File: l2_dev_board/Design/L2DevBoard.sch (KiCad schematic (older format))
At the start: 18 parts, among them P101 CONN_10X2, P102 CONN_10X2, P103 CONN_10X2, P104 CONN_10X2, P105 CONN_10X2, P106 CONN_10X2, P107 CONN_10X2, P108 CONN_10X2, P109 CONN_10X2, P110 CONN_10X2, P111 CONN_10X2, P112 CONN_10X2, P113 CONN_10X2, P114 CONN_10X2, P115 CONN_10X2, U101 ASE_20MHZ

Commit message: missing header connector for 2 L2s. Find space!
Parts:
- added P?: CONN_10X2, symbol CONN_10X2
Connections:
- net GND: now also P102.19 (P19), P103.19 (P19), P108.19 (P19), P112.19 (P19), P113.11 (P11), P113.13 (P13), P113.15 (P15), P113.17 (P17), P113.19 (P19), P113.3 (P3), P113.5 (P5), P113.7 (P7), P113.9 (P9), P114.19 (P19), P115.1 (P1), P?.1 (P1), P?.11 (P11), P?.13 (P13), P?.15 (P15), P?.17 (P17), P?.19 (P19), P?.3 (P3), P?.5 (P5), P?.7 (P7), P?.9 (P9)
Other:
- moved on the sheet: P112, P113

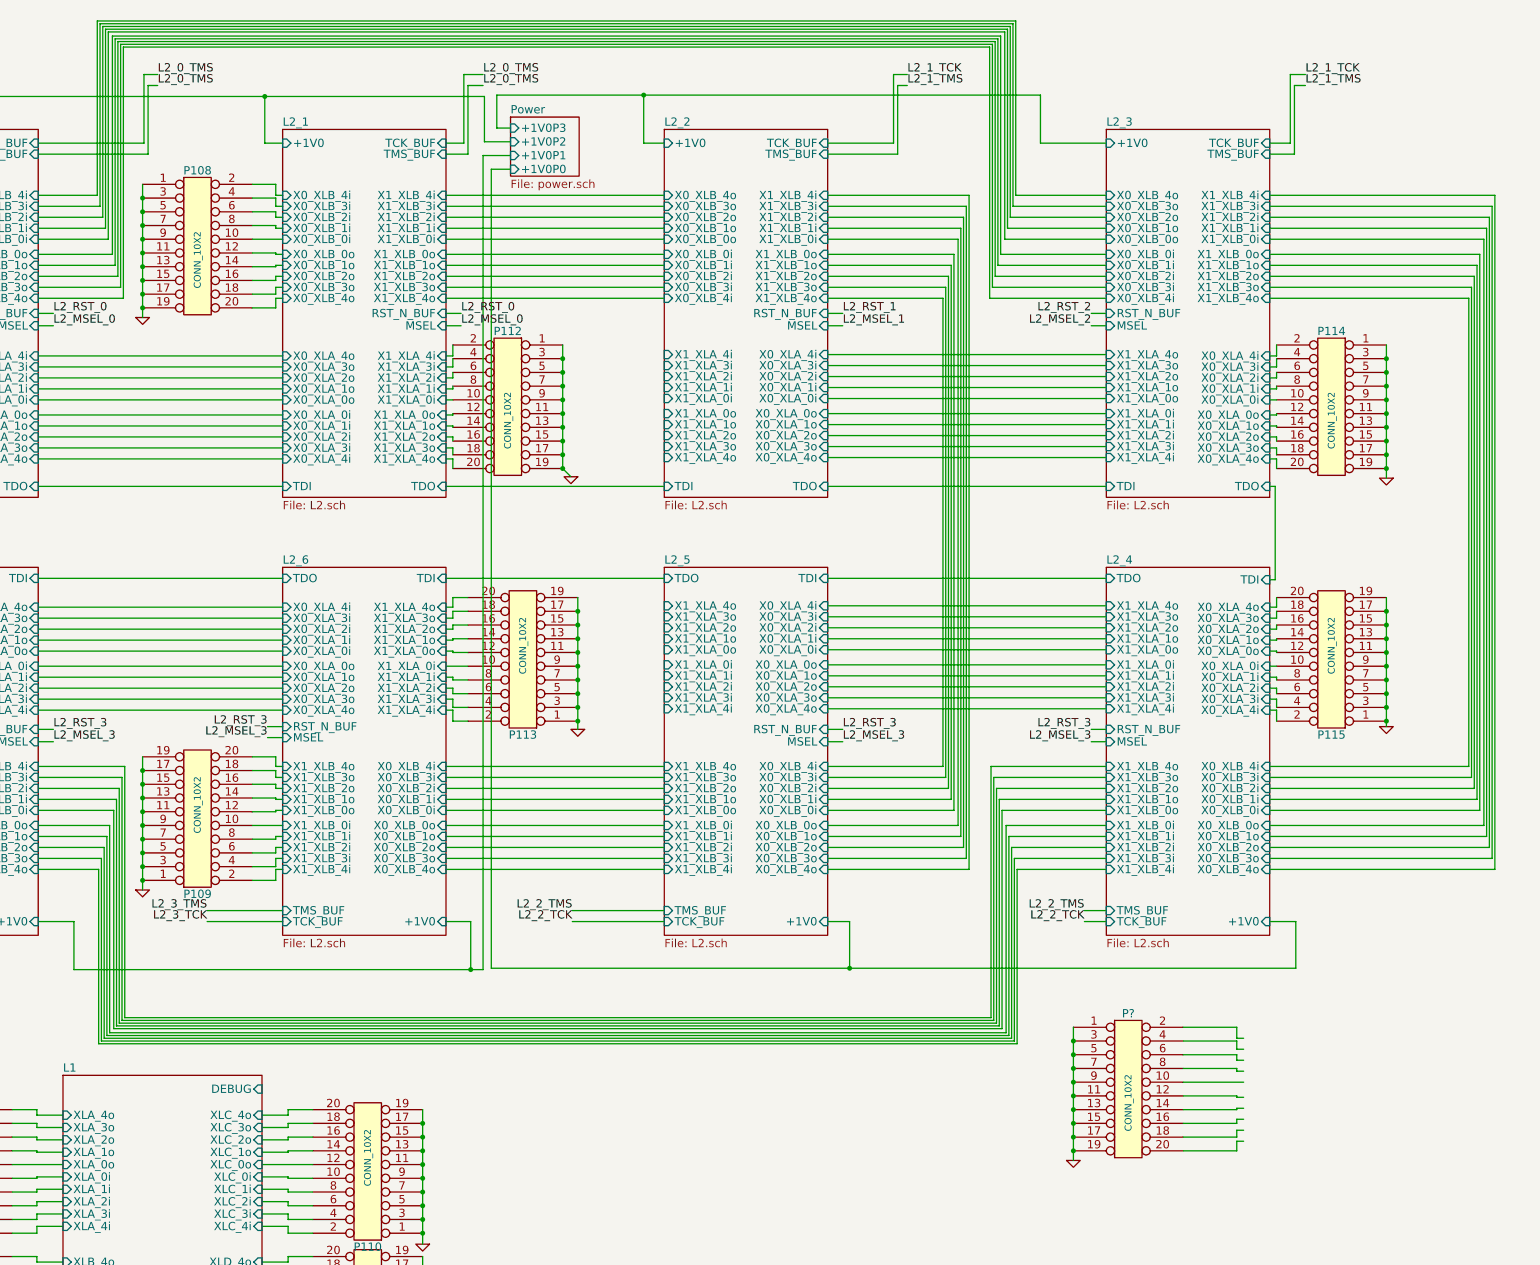
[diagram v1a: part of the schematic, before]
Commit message: workaround found for headers problem. Early start, good progess!
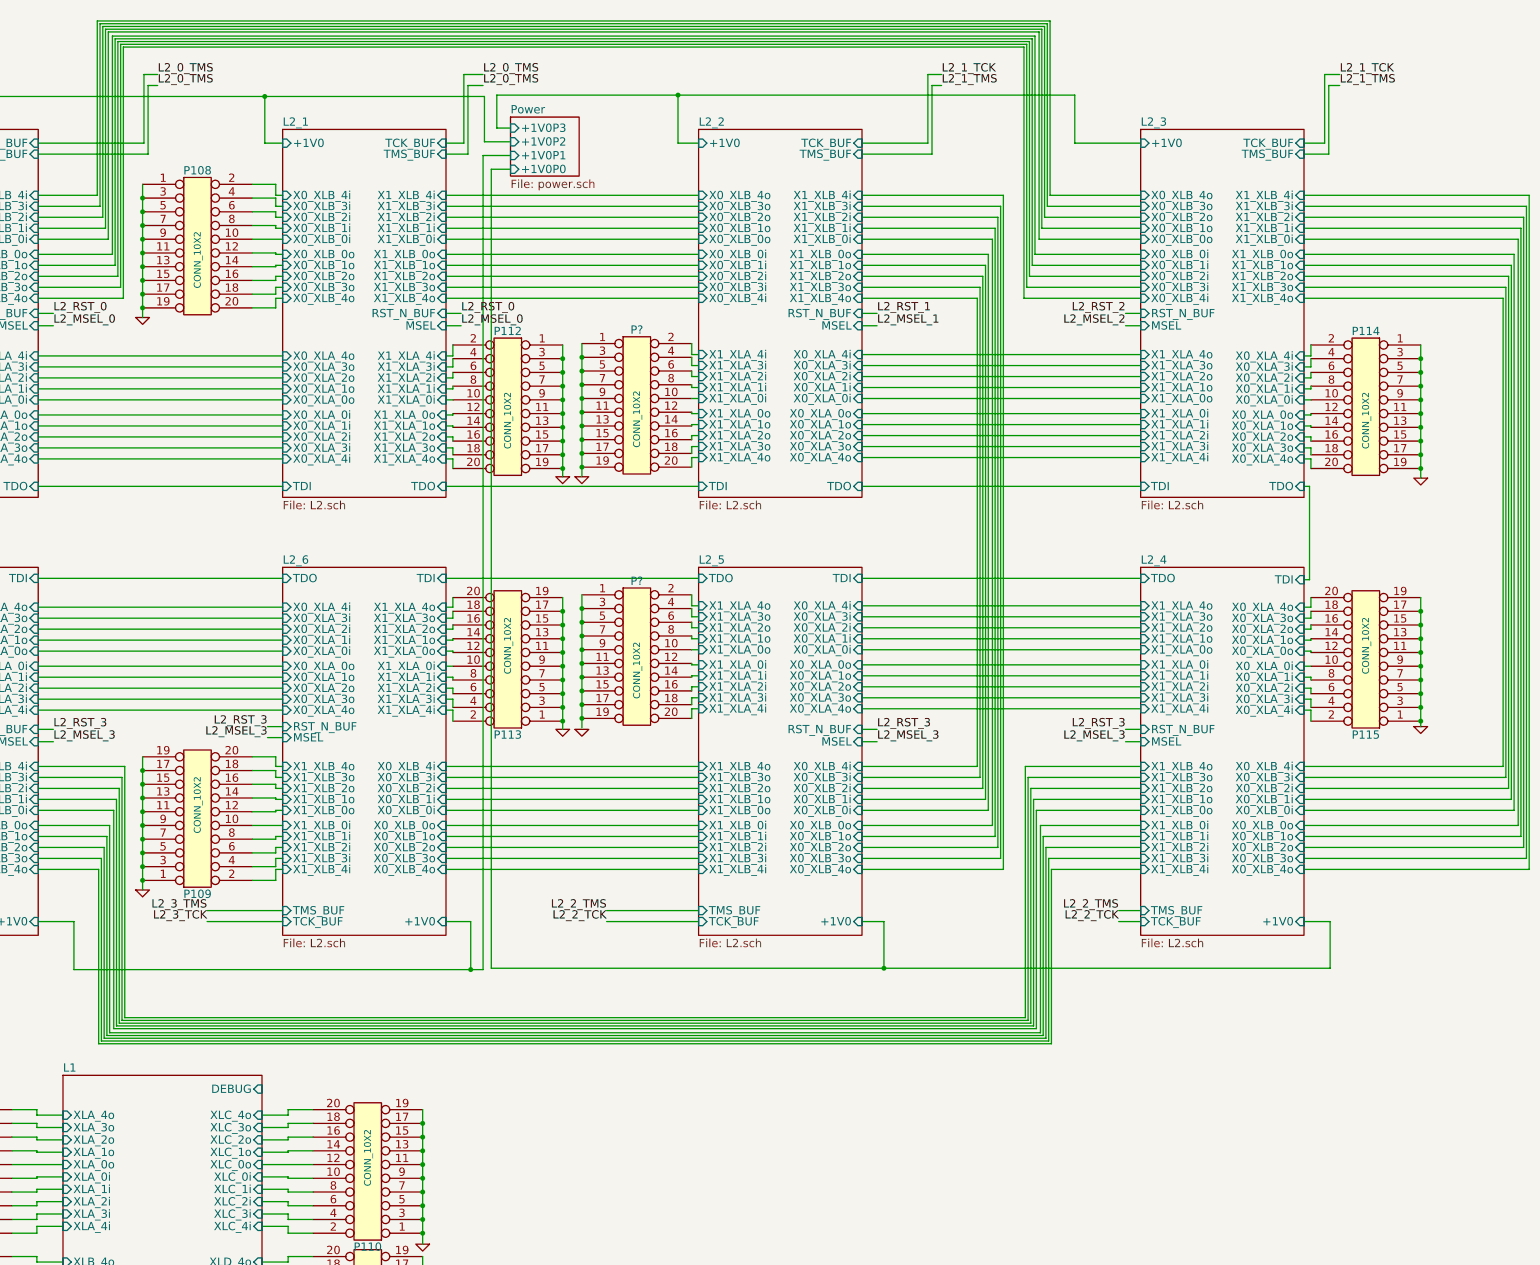
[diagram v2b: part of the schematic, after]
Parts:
- added P?: CONN_10X2, symbol CONN_10X2
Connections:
- net L2_2/X1_XLA_0i: now also P?.10 (P10)
- net L2_2/X1_XLA_0o: now also P?.12 (P12)
- net L2_2/X1_XLA_1i: now also P?.8 (P8)
- net L2_2/X1_XLA_1o: now also P?.14 (P14)
- net L2_2/X1_XLA_2i: now also P?.6 (P6)
- net L2_2/X1_XLA_2o: now also P?.16 (P16)
- net L2_2/X1_XLA_3i: now also P?.4 (P4)
- net L2_2/X1_XLA_3o: now also P?.18 (P18)
- net L2_2/X1_XLA_4i: now also P?.2 (P2)
- net L2_2/X1_XLA_4o: now also P?.20 (P20)
- net L2_5/X1_XLA_0i: now also P?.12 (P12)
- net L2_5/X1_XLA_0o: now also P?.10 (P10)
- net L2_5/X1_XLA_1i: now also P?.14 (P14)
- net L2_5/X1_XLA_1o: now also P?.8 (P8)
- net L2_5/X1_XLA_2i: now also P?.16 (P16)
- net L2_5/X1_XLA_2o: now also P?.6 (P6)
- net L2_5/X1_XLA_3i: now also P?.18 (P18)
- net L2_5/X1_XLA_3o: now also P?.4 (P4)
- net L2_5/X1_XLA_4i: now also P?.20 (P20)
- net L2_5/X1_XLA_4o: now also P?.2 (P2)
- new net: P?.1 (P1), P?.11 (P11), P?.13 (P13), P?.15 (P15), P?.17 (P17), P?.19 (P19), P?.3 (P3), P?.5 (P5), P?.7 (P7), P?.9 (P9)
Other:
- moved on the sheet: P113, P114, P115, P?
